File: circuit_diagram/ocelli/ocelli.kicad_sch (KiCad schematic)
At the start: 113 parts

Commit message: 回路図PDF追加
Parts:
- removed Y?: Crystal_GND2, symbol Device:Crystal_GND2
- removed Y?: Crystal_GND24, symbol Device:Crystal_GND24
- added R28, R5, R6: 10k, symbol Device:R
- FB1: renamed from FB?; value FerriteBead -> MZ1608-102Y
- gave numbers to parts that had none: 110
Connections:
- net 3.3_L is gone; now on net 3.3V_L: U2.14 (WM)
- net 3.3_R is gone; now on net 3.3V_R: U3.14 (WM)
- net CS_IMU is gone; now on net SPI1_CS: U4.22 (nCS)
- net CS_L is gone; now on net SPI2_CS0: J1.5 (Pin_5)
- net CS_R is gone; now on net SPI2_CS1: J2.5 (Pin_5)
- net LEFT_FRONT is gone; now on net LEFT_FRONT_IR: R25.1
- net LEFT_SIDE is gone; now on net LEFT_SIDE_IR: R11.2
- net RIGHT_FRONT is gone; now on net RIGHT_FRONT_IR: R16.1
- net RIGHT_SIDE is gone; now on net RIGHT_SIDE_IR: R1.2
- net SW_3 is gone; now on net SW_2: R32.2, SW4.1, SW4.2
- net +3.3V: now also C30.2, R28.1, R5.1, R6.1; no longer C30.1
- net BUZZER: now also U5.57 (PB5)
- net DIR_L: now also U5.43 (PA10)
- net DIR_R: now also U5.44 (PA11)
- net GND: now also C30.1; no longer C30.2
- net LED0: now also U5.40 (PC9)
- net LED1: now also U5.39 (PC8)
- net LED2: now also U5.38 (PC7)
- net LED3: now also U5.37 (PC6)
- net LEFT_FRONT_AD: now also U5.26 (PB0)
- net LEFT_SIDE_AD: now also U5.27 (PB1)
- net PWM_L: now also U5.41 (PA8)
- net PWM_R: now also U5.42 (PA9)
- net RIGHT_FRONT_AD: now also U5.25 (PC5)
- net RIGHT_SIDE_AD: now also U5.24 (PC4)
- net SW_1: now also R31.2, SW3.1, SW3.2, U5.35 (PB14); no longer R24.2, SW2.1, SW2.2
- net SW_2: now also U5.34 (PB13); no longer R31.2, SW3.1, SW3.2
- net UART_RX: now also U5.17 (PA3)
- net UART_TX: now also U5.16 (PA2)
- net VBAT_AD: now also U5.8 (PC0)
- net SPI2_MISO: now reaches U5.10 (PC2)
- net SPI2_MISO: now also J1.3 (Pin_3), J2.3 (Pin_3)
- net SPI2_MOSI: now reaches U5.11 (PC3)
- net SPI2_MOSI: now also J1.2 (Pin_2), J2.2 (Pin_2)
- net RIGHT_SIDE_IR: now reaches U5.14 (PA0)
- net RIGHT_FRONT_IR: now reaches U5.15 (PA1)
- net SPI2_CS1: now reaches U5.2 (PC13)
- net SPI2_CS1: now also R6.2
- net SPI1_CS: now reaches U5.20 (PA4)
- net SPI1_CS: now also R28.2
- net SPI1_SCLK: now reaches U5.21 (PA5)
- net SPI1_SCLK: now also U4.23 (SCL/SCLK)
- net SPI1_MISO: now reaches U5.22 (PA6)
- net SPI1_MISO: now also U4.9 (SDO/AD0)
- net SPI1_MOSI: now reaches U5.23 (PA7)
- net SPI1_MOSI: now also U4.24 (SDA/SDI)
- net SPI2_SCLK: now reaches U5.29 (PB10)
- net SPI2_SCLK: now also J1.4 (Pin_4), J2.4 (Pin_4)
- net LEFT_FRONT_IR: now reaches U5.30 (PB11)
- net LEFT_SIDE_IR: now reaches U5.33 (PB12)
- net SW_0: now reaches U5.36 (PB15)
- net SW_0: now also R24.2, SW2.1, SW2.2
- net SPI2_CS0: now reaches U5.9 (PC1)
- net SPI2_CS0: now also R5.2
- removed net MISO: J1.3 (Pin_3), J2.3 (Pin_3), U4.9 (SDO/AD0)
- removed net MOSI: J1.2 (Pin_2), J2.2 (Pin_2), U4.24 (SDA/SDI)
- removed net SCLK: J1.4 (Pin_4), J2.4 (Pin_4), U4.23 (SCL/SCLK)
- no-connect marks 9 -> 24
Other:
- note added: "Buzzer"
- note added: "Encoder"
- note added: "LED"
- note added: "Micon"
- note added: "Power"
- note added: "Switch"
- moved on the sheet: BT1, C1, C10, C11, C12, C13, C14, C15, C16, C17, C18, C19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

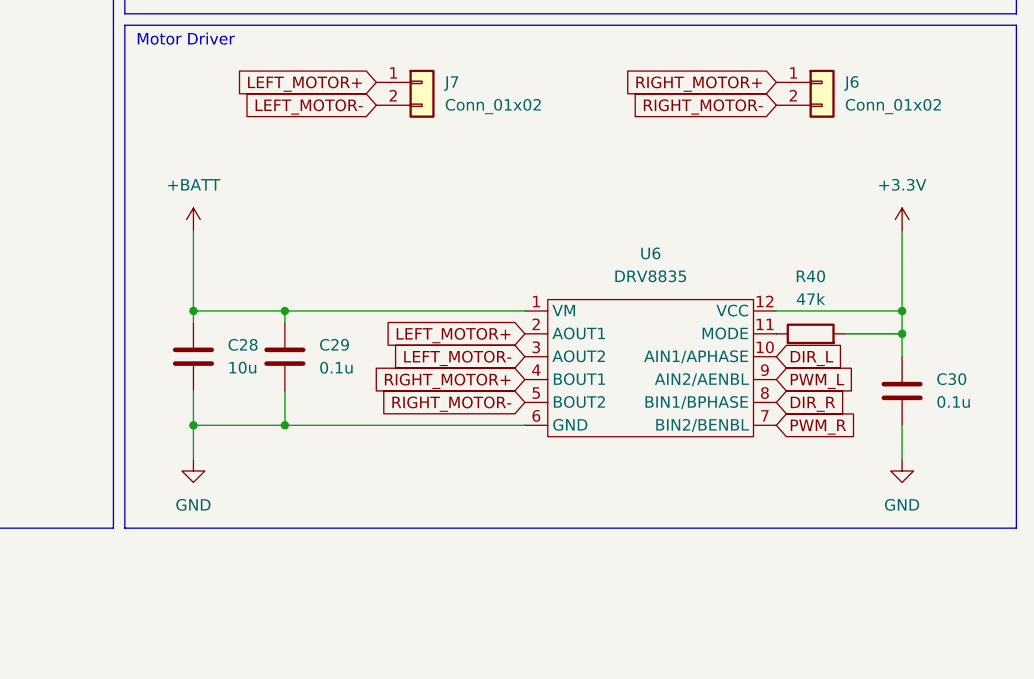
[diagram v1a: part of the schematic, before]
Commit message: スタイル調整
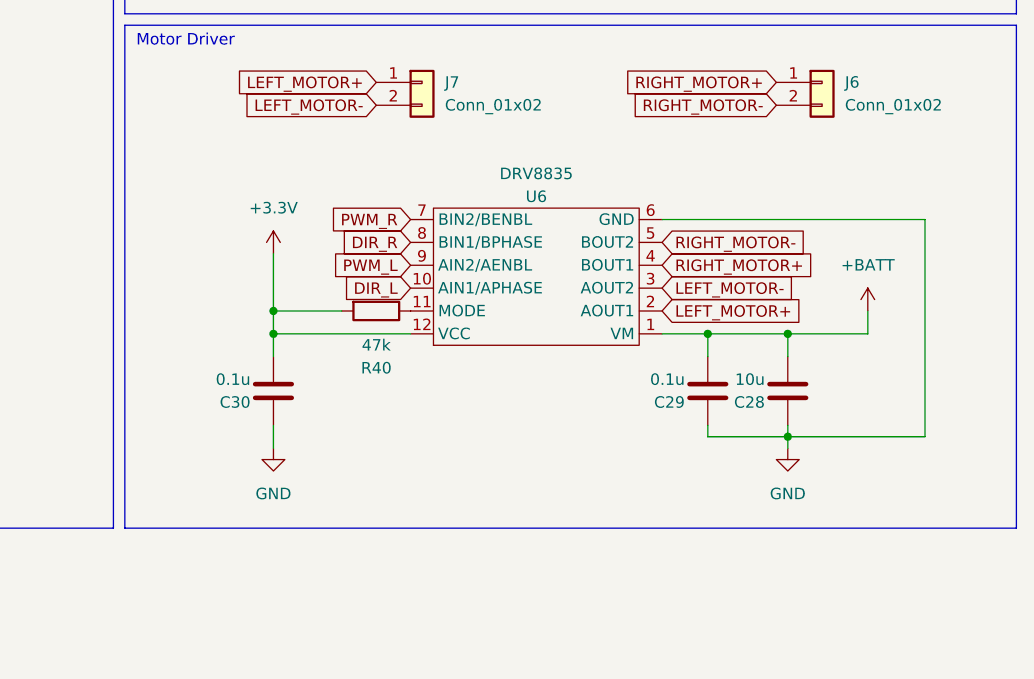
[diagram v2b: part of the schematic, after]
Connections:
- net +3.3V: now also C30.1; no longer C30.2
- net +BATT: now also C28.1, C29.1; no longer C28.2, C29.2
- net GND: now also C28.2, C29.2, C30.2; no longer C28.1, C29.1, C30.1
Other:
- moved on the sheet: C28, C29, C30, R40, U6
